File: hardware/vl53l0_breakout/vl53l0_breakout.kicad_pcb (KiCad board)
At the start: 2 copper layers, 15 parts, among them J1 Conn_01x06, U1 VL53L0CXV0DH1

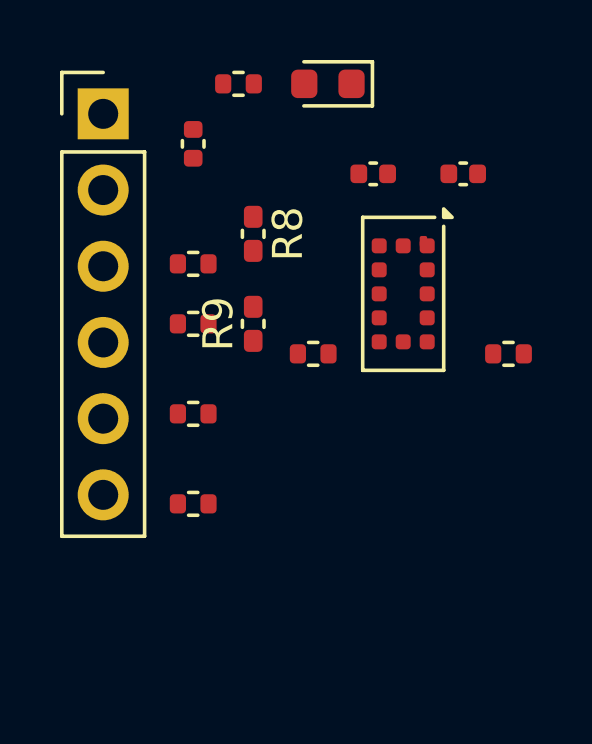
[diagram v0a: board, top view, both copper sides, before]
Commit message: routing
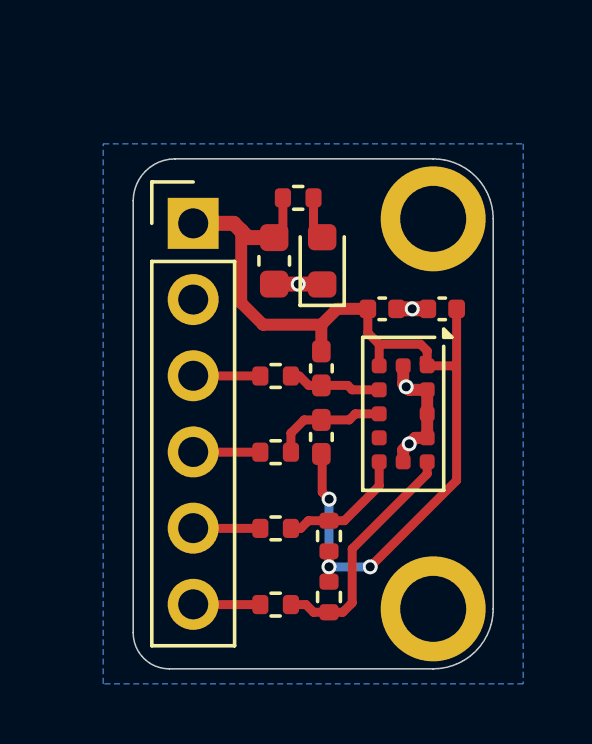
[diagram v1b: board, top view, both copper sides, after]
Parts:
- added H1: MountingHole_Pad, MountingHole:MountingHole_2.2mm_M2_ISO7380_Pad, F.Cu at (151.0, 67.5)
- added H2: MountingHole_Pad, MountingHole:MountingHole_2.2mm_M2_ISO7380_Pad, F.Cu at (151.0, 80.5)
- C3: footprint Capacitor_SMD:C_0402_1005Metric -> Capacitor_SMD:C_0603_1608Metric
- moved R7 10.1 mm to (147.5, 80.1), turned to -90 degrees
- moved R1 6.09 mm to (147.5, 78.1), turned to 90 degrees
- moved D2 5.90 mm to (147.3, 68.9), turned to 90 degrees
- moved R4 5.08 mm to (145.7, 75.3)
- moved R8 5.03 mm to (147.3, 72.5)
- moved C3 4.74 mm to (145.7, 68.9)
- moved J1 4.72 mm to (143.0, 67.7)
- moved R5 4.70 mm to (145.7, 77.8)
- moved R3 4.64 mm to (145.7, 72.7)
- moved C2 4.55 mm to (151.3, 70.5), turned to 180 degrees
- moved C1 4.51 mm to (149.3, 70.5)
- moved R9 4.40 mm to (147.3, 74.8)
- moved R6 4.34 mm to (145.7, 80.4)
- moved R2 4.29 mm to (146.5, 66.8)
- moved U1 4.00 mm to (150.0, 74.0)
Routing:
- net +3.3V: track 0.00 -> 33.3 mm, vias 0 -> 3
- net /TOF_XSHUT: track 0.00 -> 8.01 mm
- net GND: track 0.00 -> 7.09 mm, vias 0 -> 4
- net /TOF_GPIO1: track 0.00 -> 4.33 mm
- net /TOF_I2C_SDA: track 0.00 -> 3.84 mm
- net /TOF_I2C_SCL: track 0.00 -> 3.13 mm
- net /XSHUT: track 0.00 -> 2.24 mm
- net /I2C_SDA: track 0.00 -> 2.24 mm
- net /I2C_SCL: track 0.00 -> 2.24 mm
- net /GPIO1: track 0.00 -> 2.24 mm
- net /LEDK: track 0.00 -> 1.43 mm
- added copper zone on B.Cu, net GND
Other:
- board outline added: 12 x 17 mm
- board text added: "3.3V"
- board text added: "GND"
- board text added: "GPIO1"
- board text added: "SCL"
- board text added: "SDA"
- board text added: "VL53L0 CXV0DH1"
- board text added: "XST"
